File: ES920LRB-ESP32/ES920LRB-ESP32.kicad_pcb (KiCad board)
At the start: 2 copper layers, 15 parts, among them J1 Conn_01x19_Female, J2 Conn_01x19_Female, J3 Conn_01x13_Female, J4 Conn_01x13_Female, M1 ES920LR2B, U1 ESP32-DEVKITC-32D

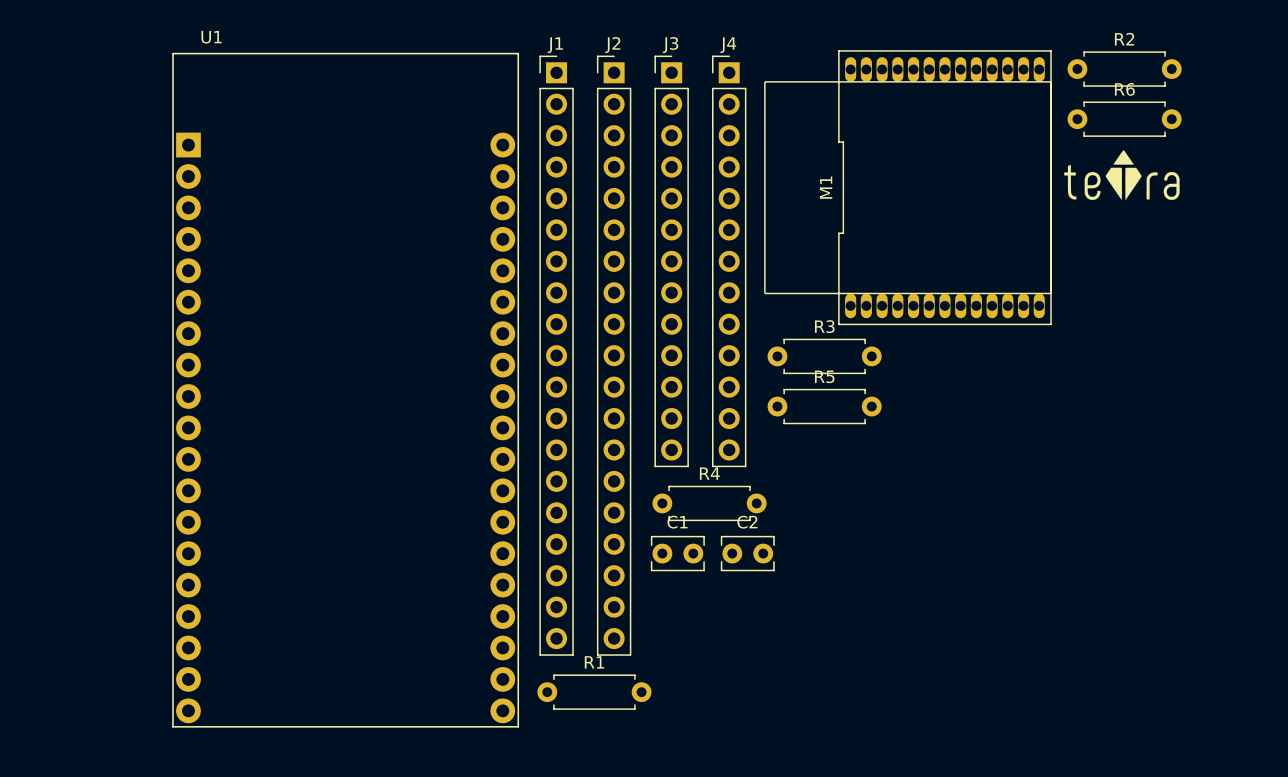
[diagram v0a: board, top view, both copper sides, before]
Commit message: add ES920LRB-ESP32 v1.4
add ES920LRB-ESP32 v1.4
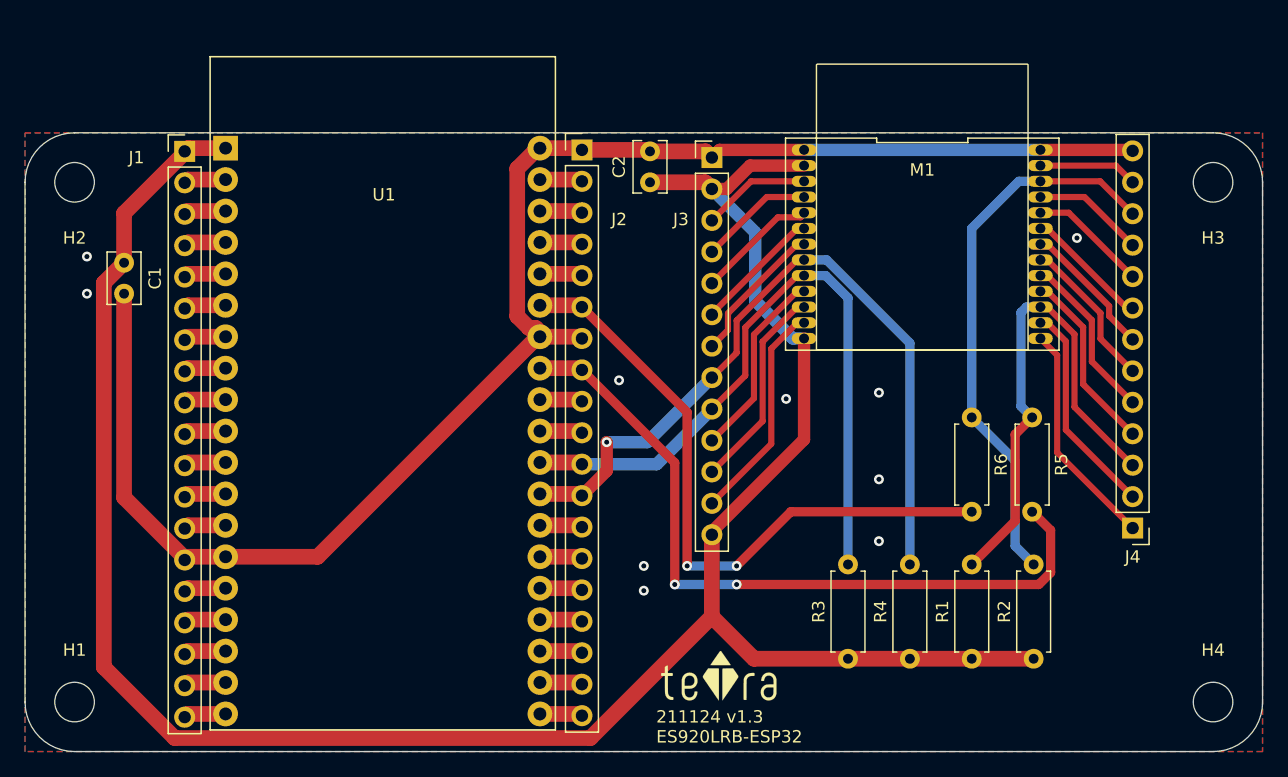
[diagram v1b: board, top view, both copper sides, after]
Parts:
- added H1: MountingHole, MountingHole:MountingHole_3.2mm_M3, F.Cu at (101.0, 139.0)
- added H2: MountingHole, MountingHole:MountingHole_3.2mm_M3, F.Cu at (101.0, 97.0)
- added H3: MountingHole, MountingHole:MountingHole_3.2mm_M3, F.Cu at (193.0, 97.0)
- added H4: MountingHole, MountingHole:MountingHole_3.2mm_M3, F.Cu at (193.0, 139.0)
- moved L1 51.9 mm to (153.0, 138.0)
- moved C1 49.4 mm to (105.0, 103.5), turned to 270 degrees
- moved J4 49.2 mm to (186.5, 124.9), turned to 180 degrees
- moved R2 47.8 mm to (178.5, 135.5), turned to 90 degrees
- moved R1 34.4 mm to (173.5, 135.5), turned to 90 degrees
- moved C2 30.7 mm to (147.5, 97.0), turned to 90 degrees
- moved J1 30.7 mm to (109.9, 94.5)
- moved R6 25.6 mm to (173.5, 116.0), turned to 270 degrees
- moved R3 25.1 mm to (163.5, 135.5), turned to 90 degrees
- moved R4 23.6 mm to (168.5, 135.5), turned to 90 degrees
- moved R5 20.6 mm to (178.4, 116.0), turned to 270 degrees
- moved J3 7.58 mm to (152.5, 95.0)
- moved J2 6.75 mm to (142.0, 94.4)
- moved M1 4.92 mm to (169.5, 102.0), turned to 270 degrees
- moved U1 3.01 mm to (125.9, 114.0)
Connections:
- R1 pad 2: Net-(J2-Pad8) -> ES920_WKUP1
- R2 pad 2: Net-(J2-Pad6) -> ES920_NRST
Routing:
- net +3V3: track 0.00 -> 185.5 mm
- net GND: track 0.00 -> 128.9 mm, vias 0 -> 10
- net Host_RX-ES920_TX: track 0.00 -> 61.4 mm, vias 0 -> 1
- net Net-(J2-Pad8): track 0.00 -> 60.2 mm, vias 0 -> 2
- net Host_TX-ES920RX: track 0.00 -> 55.8 mm
- net Net-(J2-Pad6): track 0.00 -> 52.7 mm, vias 0 -> 2
- net ES920_NRST: track 0.00 -> 44.9 mm
- net ES920_WKUP1: track 0.00 -> 40.7 mm
- net Net-(J4-Pad1): track 0.00 -> 18.4 mm
- net Net-(J3-Pad12): track 0.00 -> 18.0 mm
- net Net-(J4-Pad2): track 0.00 -> 17.5 mm
- net Net-(J3-Pad11): track 0.00 -> 16.7 mm
- net Net-(J3-Pad10): track 0.00 -> 15.5 mm
- net Net-(J4-Pad4): track 0.00 -> 14.9 mm
- net Net-(J4-Pad5): track 0.00 -> 13.6 mm
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- added copper zone on B.Cu, net GND
- added copper zone on F.Cu, net GND
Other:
- board outline added: 100 x 50 mm
- board text added: "211124 v1.3 ES920LRB-ESP32"
